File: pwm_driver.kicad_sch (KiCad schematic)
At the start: 41 parts, among them J1 V_{In}, J2 GND_{In}, J3 SolderPad, J4 SolderPad, Q1 BC817, Q2 BC807, Q3 BUK7880-55A, U1 TLV2372, U2 LM393

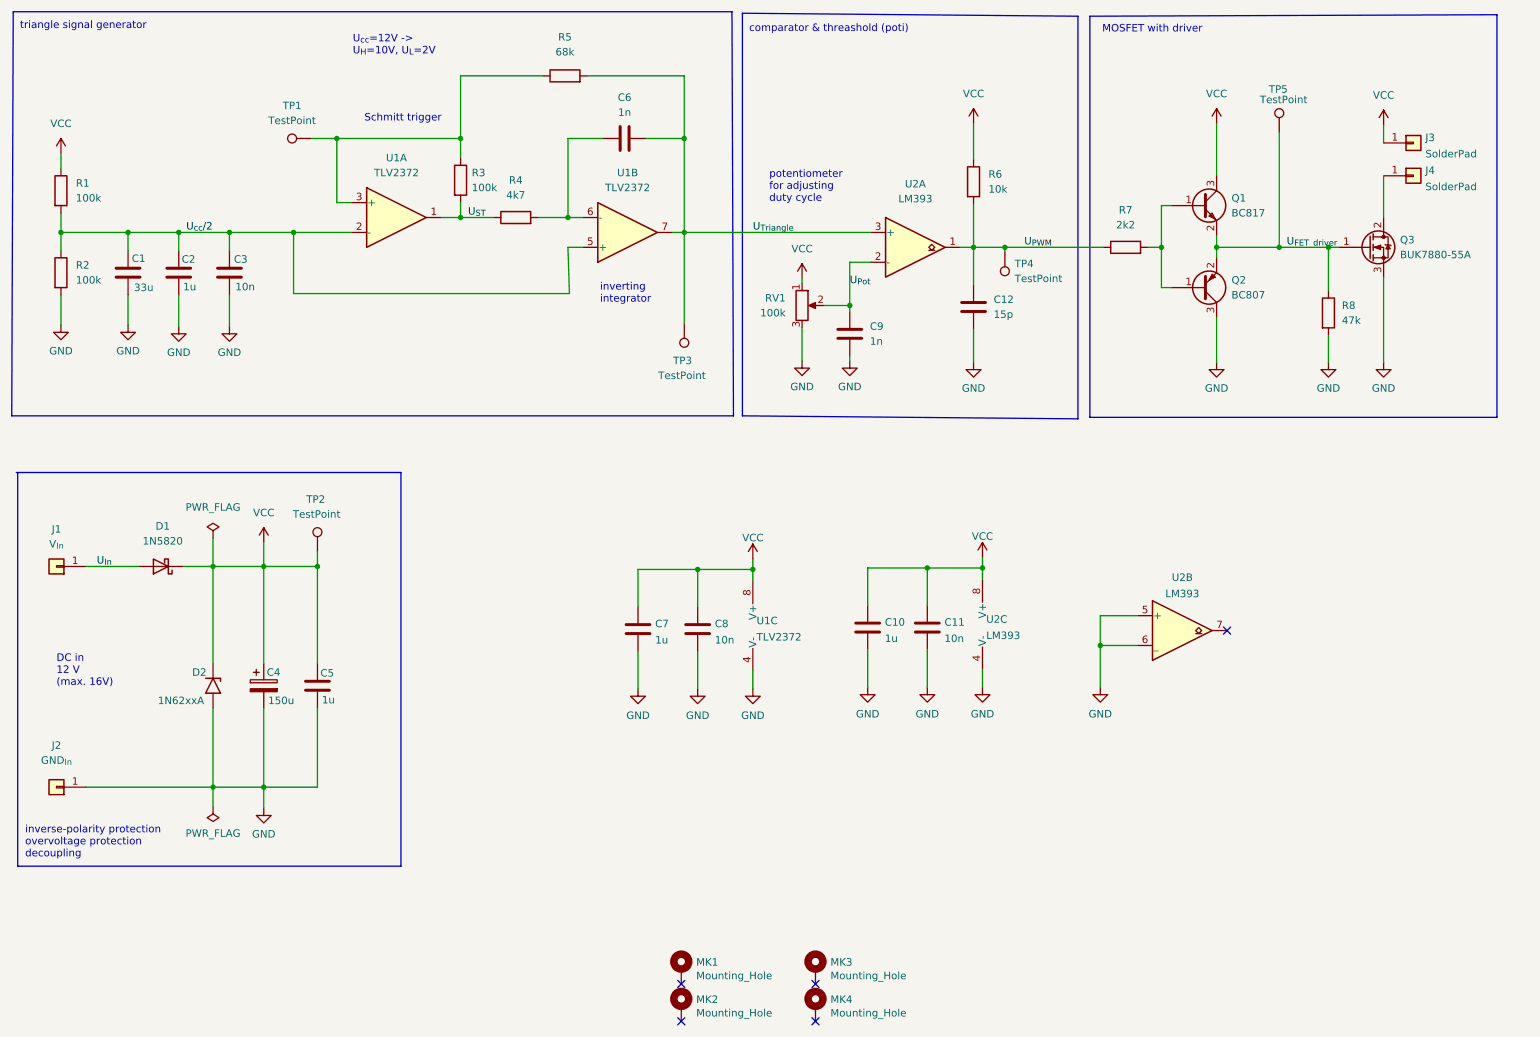
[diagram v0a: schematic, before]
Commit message: photo added from working device
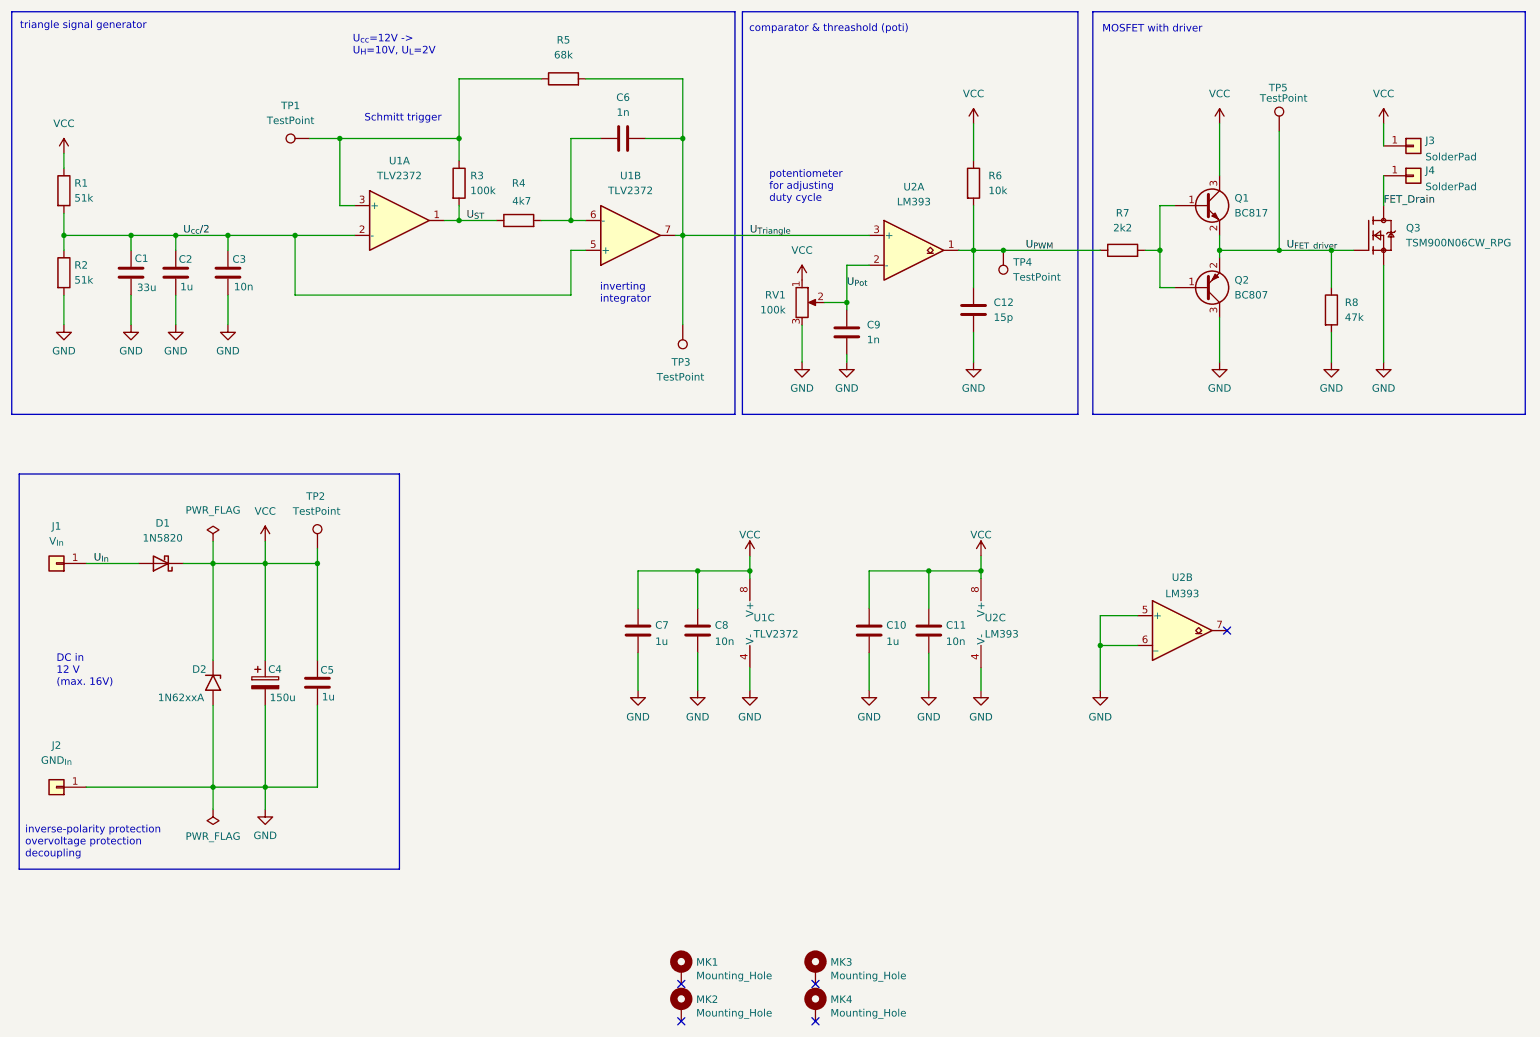
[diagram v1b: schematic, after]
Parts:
- removed Q3: BUK7880-55A, Package_TO_SOT_SMD:SOT-223-3_TabPin2, symbol Transistor_FET:BUK7880-55A
- added Q3: TSM900N06CW_RPG, TRANS_TSM900N06CW_RPG:TRANS_TSM900N06CW_RPG, symbol TSM900N06CW_RPG:TSM900N06CW_RPG
- R1, R2: value 100k -> 51k
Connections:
- net GND: now also Q3.3
- net U_{FET_driver}: now also Q3.1
- net FET_Drain: now reaches J4.1 (Pin_1)
- net FET_Drain: now also Q3.2, Q3.4
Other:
- moved on the sheet: C1, C10, C11, C12, C2, C4, C5, C9, D1, D2, J1, J3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
